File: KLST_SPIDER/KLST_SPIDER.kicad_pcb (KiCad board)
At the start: 2 copper layers, 139.5 x 46.5 mm, 25 parts, among them J1 MIDI_IN, J10 UART, J11 UART, J12 UART, J13 MIDI_THRU, J2 MIDI_OUT, J3 UART, J4 UART, J5 UART, J6 UART, J7 UART, J8 UART, J9 UART, U1 H11L1, U2 74AHC1G125, U3 74AHC1G125

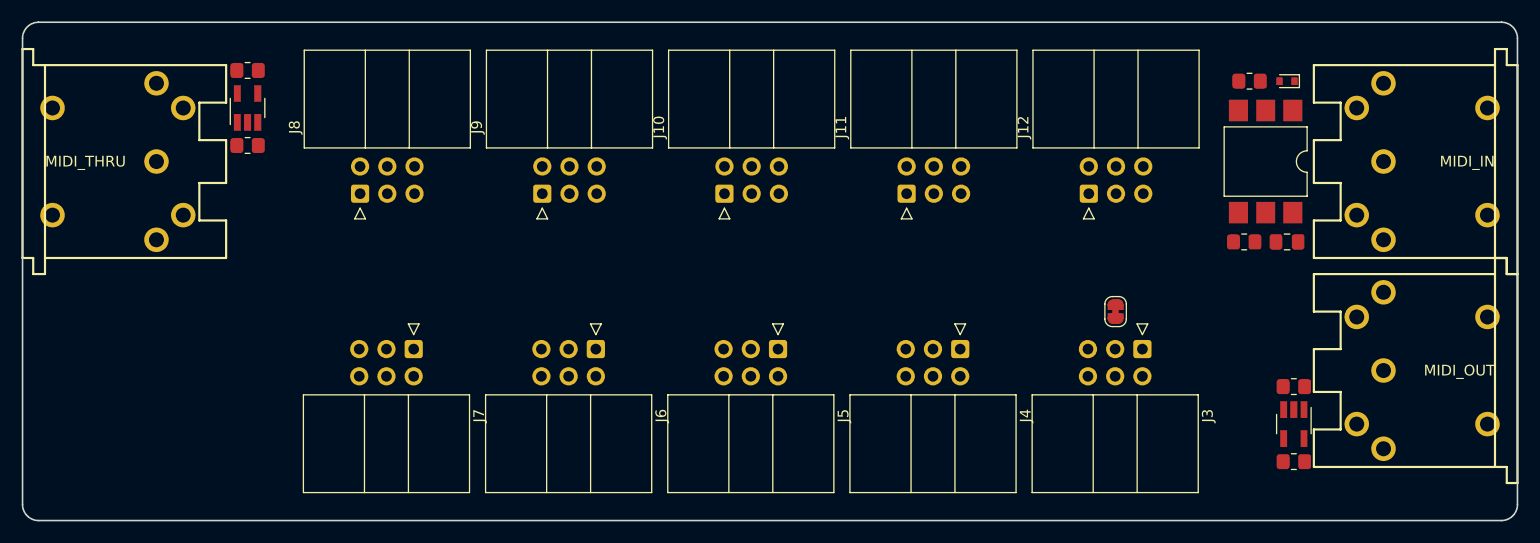
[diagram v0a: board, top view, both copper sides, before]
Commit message: prepared JLPCPB production
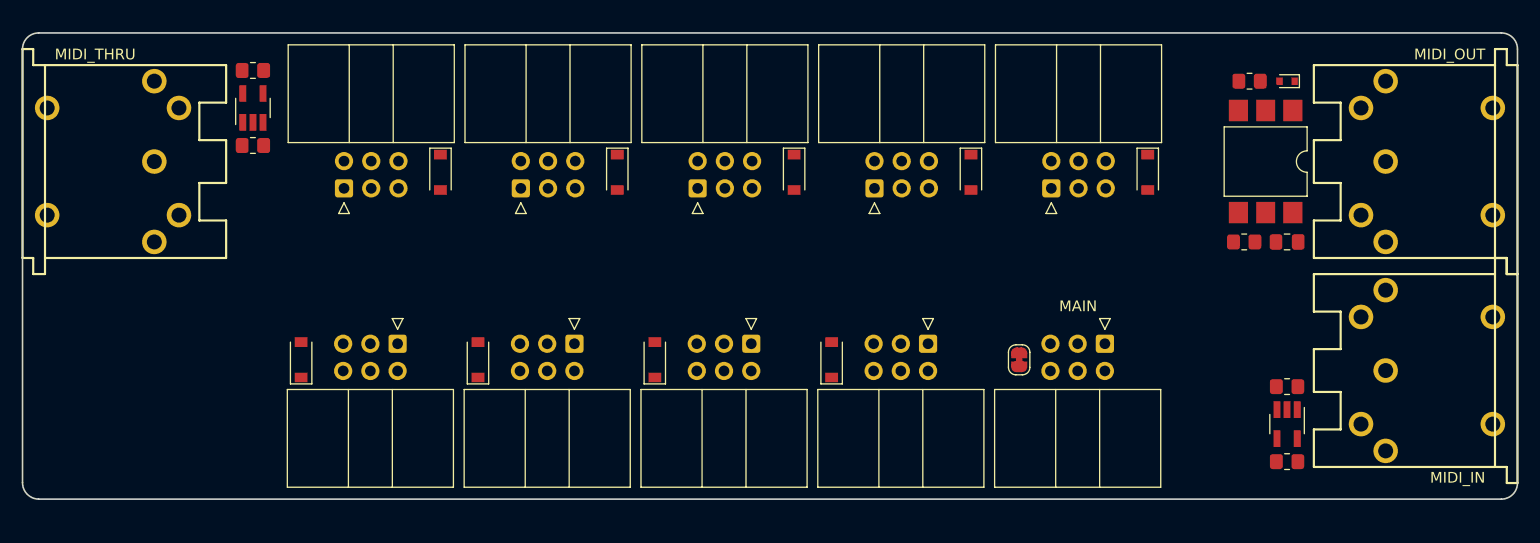
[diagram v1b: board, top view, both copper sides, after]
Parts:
- removed the J4 at (170.5, 108.5)
- added D10: Schottky, Diode_SMD:D_SOD-123, F.Cu at (122.0, 92.0)
- added D2: Schottky, Diode_SMD:D_SOD-123, F.Cu at (158.5, 109.5)
- added D3: Schottky, Diode_SMD:D_SOD-123, F.Cu at (142.0, 109.5)
- added D4: Schottky, Diode_SMD:D_SOD-123, F.Cu at (125.5, 109.5)
- added D5: Schottky, Diode_SMD:D_SOD-123, F.Cu at (109.0, 109.5)
- added D6: Schottky, Diode_SMD:D_SOD-123, F.Cu at (188.0, 92.0)
- added D7: Schottky, Diode_SMD:D_SOD-123, F.Cu at (171.5, 92.0)
- added D8: Schottky, Diode_SMD:D_SOD-123, F.Cu at (155.0, 92.0)
- added D9: Schottky, Diode_SMD:D_SOD-123, F.Cu at (138.5, 92.0)
- added J3: MIDI_THRU, DIN-5:DIN5-RA-PTH, F.Cu at (83.0, 91.0)
- J13: value MIDI_THRU -> UART; footprint DIN-5:DIN5-RA-PTH -> Connector_IDC:IDC-Header_2x03_P2.54mm_Horizontal
- U1: value H11L1 -> H11L1SR2M
- moved J12 53.0 mm to (129.5, 93.5)
- moved J9 47.5 mm to (179.0, 93.5)
- moved J13 30.1 mm to (113.0, 93.5), turned to 90 degrees
- moved J11 19.5 mm to (146.0, 93.5)
- moved J1 19.5 mm to (222.5, 110.5)
- moved J2 19.5 mm to (222.5, 91.0)
- moved J7 15.0 mm to (134.5, 108.0)
- moved J6 14.5 mm to (151.0, 108.0)
- moved J8 14.4 mm to (118.0, 108.0), turned to -90 degrees
- moved J10 14.0 mm to (162.5, 93.5)
- moved J5 14.0 mm to (167.5, 108.0)
- moved JP1 10.1 mm to (176.0, 109.5)
- moved J4 3.54 mm to (184.0, 108.0)
- moved R1 0.63 mm to (201.0, 112.0)
- moved R4 0.63 mm to (201.0, 119.0)
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- renumbered J3 to J4, R5 to R2, R2 to R3, R3 to R4, R6 to R5, R4 to R6
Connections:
- J1 pad 6: (no net) -> unconnected-(J1-Pad6)
- J1 pad 7: (no net) -> unconnected-(J1-Pad7)
- J10 pad 3: /PWR -> Net-(D7-Pad1)
- J10 pad 4: /PWR -> Net-(D7-Pad1)
- J11 pad 3: /PWR -> Net-(D8-Pad1)
- J11 pad 4: /PWR -> Net-(D8-Pad1)
- J12 pad 3: /PWR -> Net-(D9-Pad1)
- J12 pad 4: /PWR -> Net-(D9-Pad1)
- J13 pad 1: unconnected-(J13-Pad1) -> GND
- J13 pad 2: GND -> /UART_RX
- J13 pad 3: unconnected-(J13-Pad3) -> Net-(D10-Pad1)
- J13 pad 4: Net-(J13-Pad4) -> Net-(D10-Pad1)
- J13 pad 5: Net-(J13-Pad5) -> /UART_TX
- J13 pad 6: (no net) -> GND
- J2 pad 6: (no net) -> unconnected-(J2-Pad6)
- J2 pad 7: (no net) -> unconnected-(J2-Pad7)
- J5 pad 3: /PWR -> Net-(D2-Pad1)
- J5 pad 4: /PWR -> Net-(D2-Pad1)
- J6 pad 3: /PWR -> Net-(D3-Pad1)
- J6 pad 4: /PWR -> Net-(D3-Pad1)
- J7 pad 3: /PWR -> Net-(D4-Pad1)
- J7 pad 4: /PWR -> Net-(D4-Pad1)
- J8 pad 3: /PWR -> Net-(D5-Pad1)
- J8 pad 4: /PWR -> Net-(D5-Pad1)
- J9 pad 3: /PWR -> Net-(D6-Pad1)
- J9 pad 4: /PWR -> Net-(D6-Pad1)
- R2 pad 2: Net-(J13-Pad4) -> Net-(J3-Pad4)
- R5 pad 1: Net-(J13-Pad5) -> Net-(J3-Pad5)
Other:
- board size 139.5 x 46.5 mm -> 139.5 x 43.5 mm
- board text added: "MAIN"
